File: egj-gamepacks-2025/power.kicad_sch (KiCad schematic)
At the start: 13 parts, among them J1 USB_B_Micro, U13 LD1117S18TR_SOT223, U3 NCP1117-3.3_SOT223

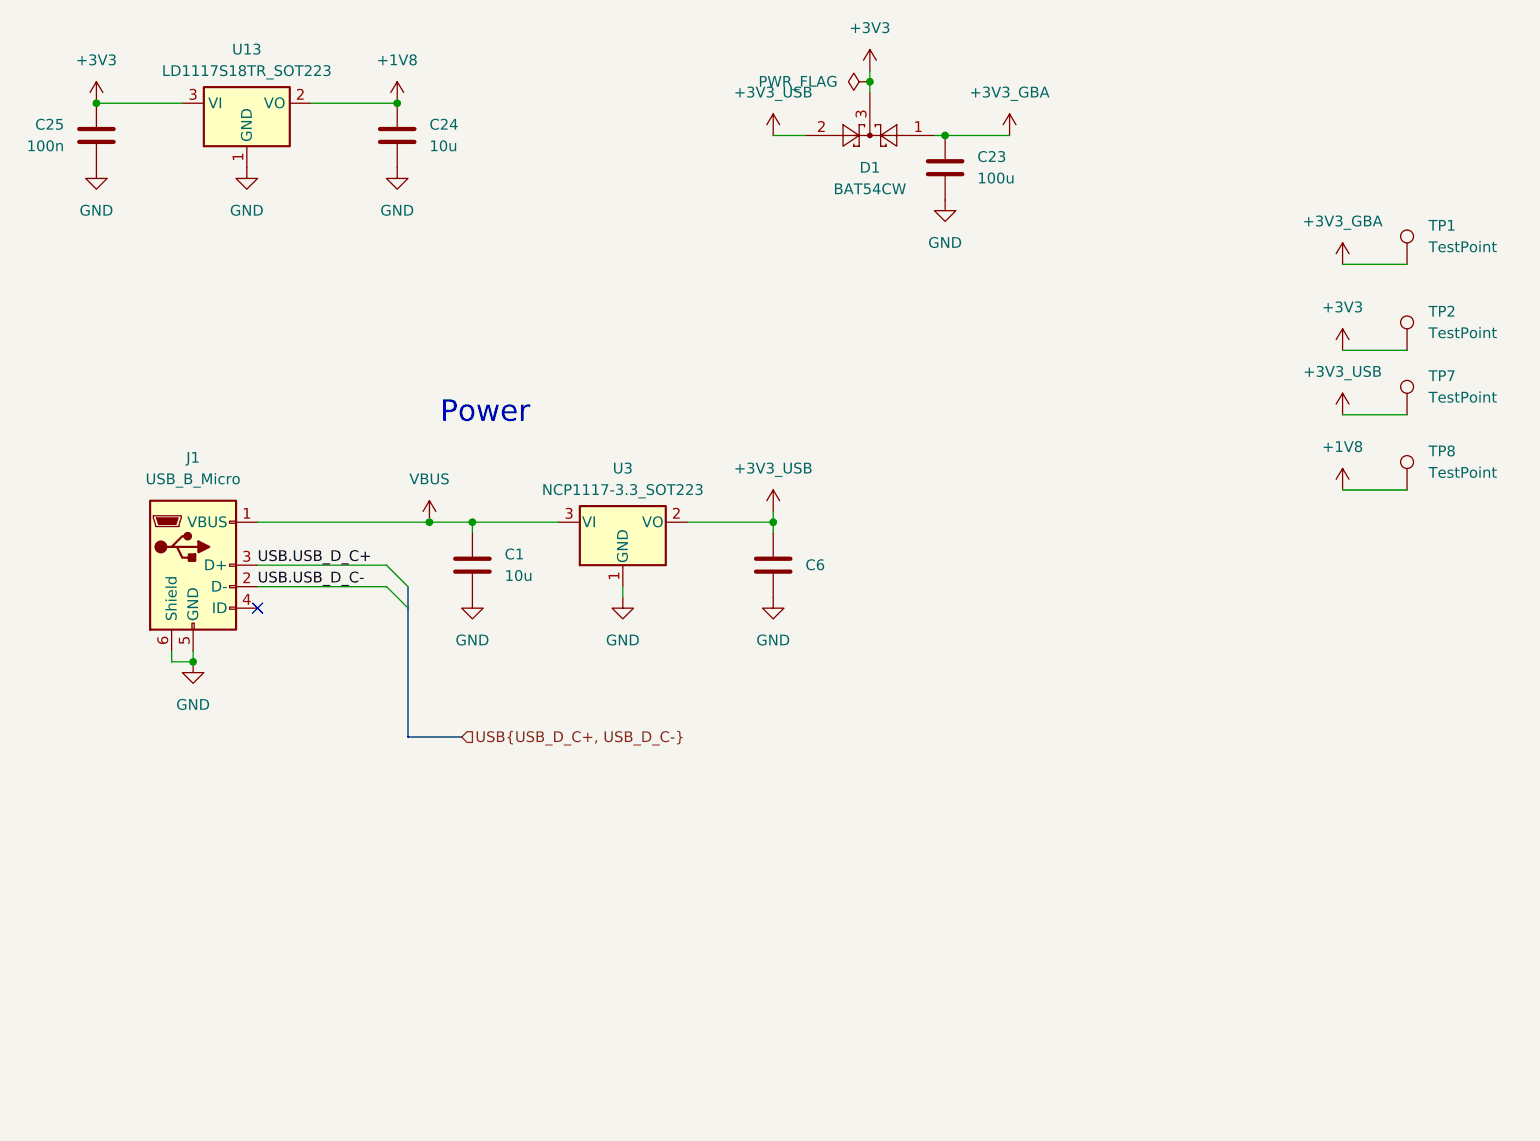
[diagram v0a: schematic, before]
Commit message: Update
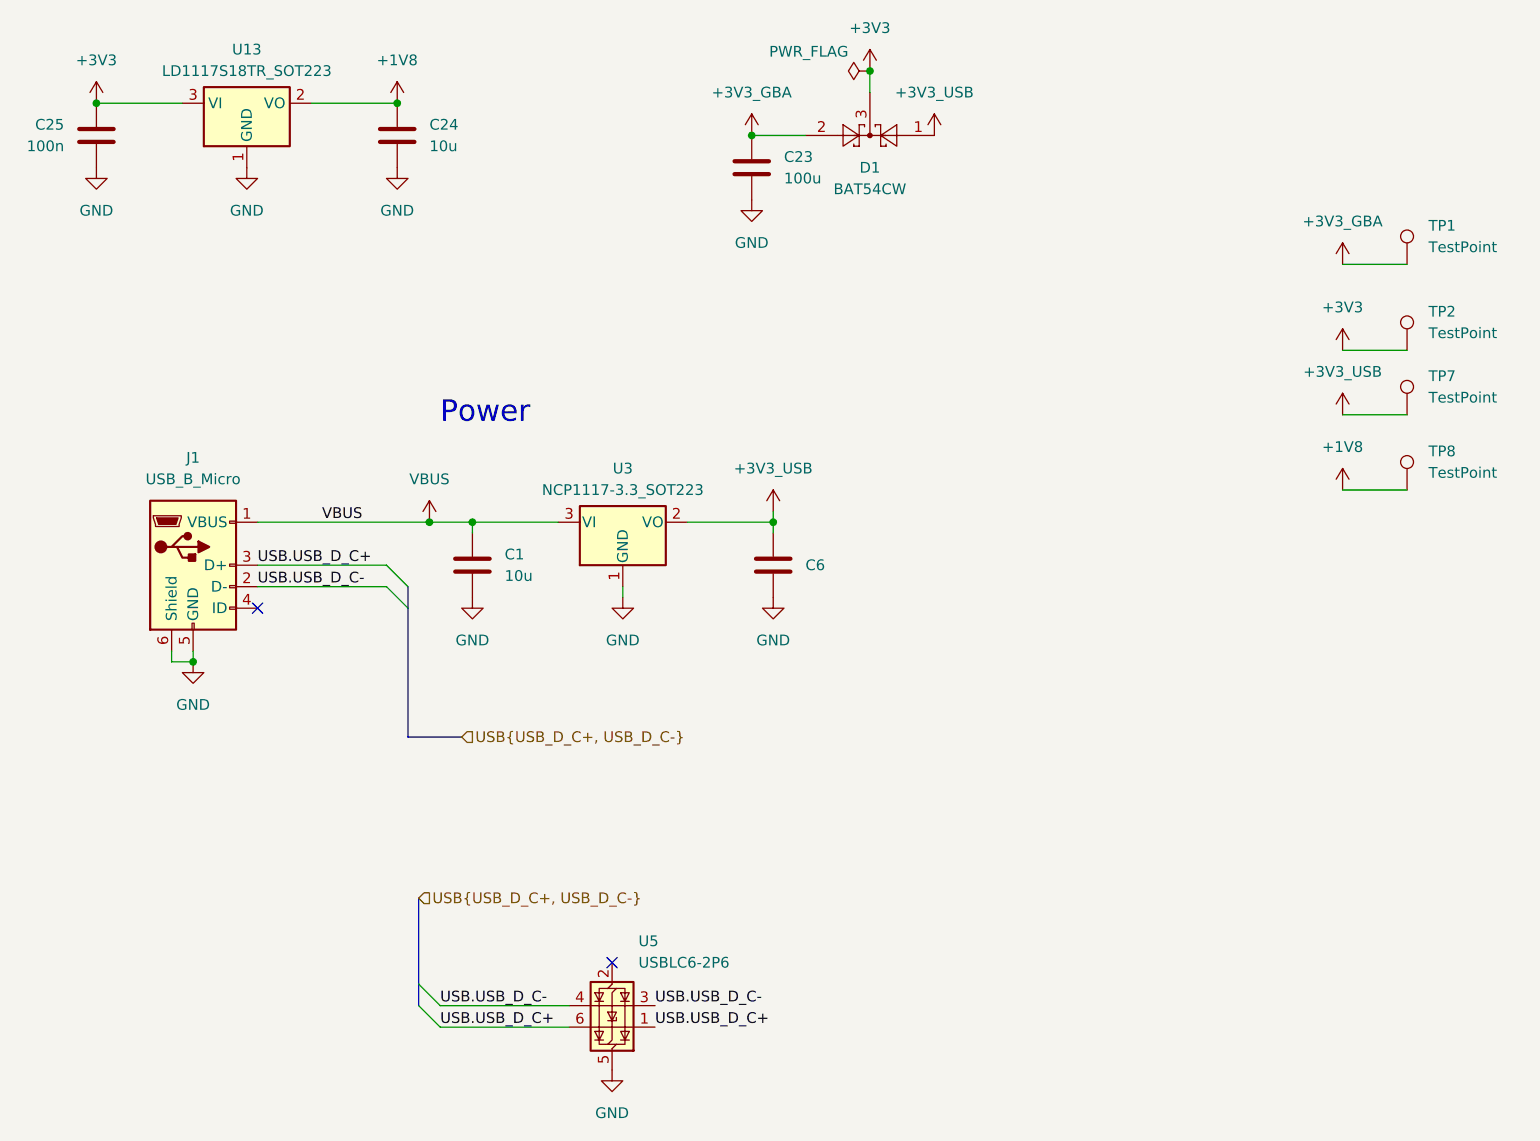
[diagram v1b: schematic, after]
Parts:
- added U5: USBLC6-2P6, Package_TO_SOT_SMD:SOT-666, symbol Power_Protection:USBLC6-2P6
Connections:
- net +3V3_GBA: now also D1.2; no longer D1.1
- net +3V3_USB: now also D1.1; no longer D1.2
- net GND: now also U5.5 (VBUS)
- net USB.USB_D_C+: now also U5.1 (I/O1), U5.6 (I/O1)
- net USB.USB_D_C-: now also U5.3 (I/O2), U5.4 (I/O2)
- no-connect marks 1 -> 2
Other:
- moved on the sheet: C23
